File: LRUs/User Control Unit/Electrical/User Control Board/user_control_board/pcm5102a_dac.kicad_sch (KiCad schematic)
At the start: 1 part

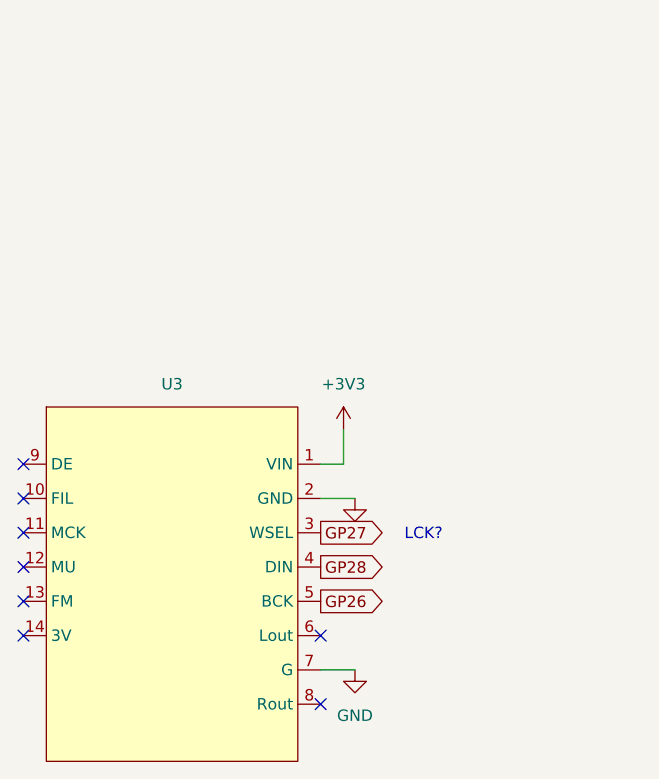
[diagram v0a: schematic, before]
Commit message: connectors and 5v buck partially done
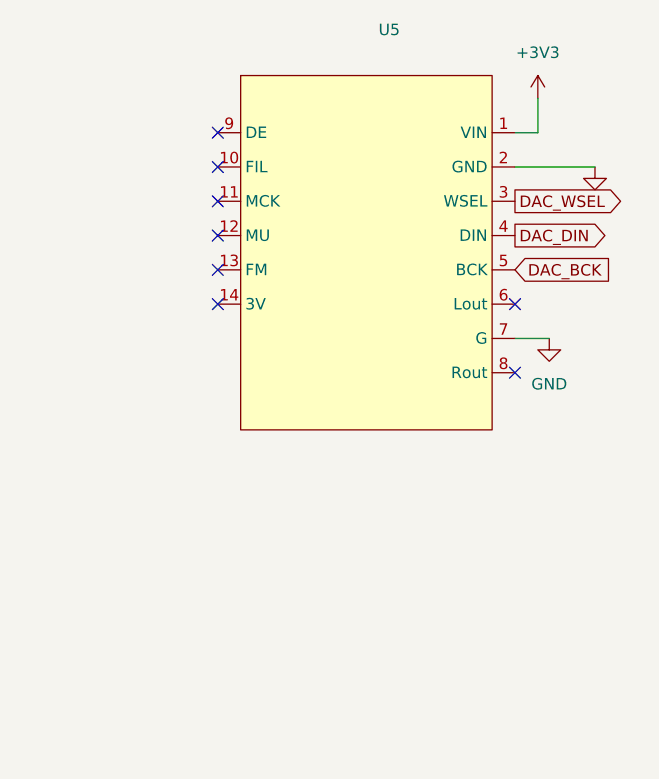
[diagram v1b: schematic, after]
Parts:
- renumbered U3 to U5
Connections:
- net GP26 renamed DAC_BCK
- net GP27 renamed DAC_WSEL
- net GP28 renamed DAC_DIN
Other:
- note removed: "LCK?"
- moved on the sheet: U5
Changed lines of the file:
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@@
 	(generator_version "10.0")
 	(paper "A4")
-	(text "LCK?"
+	(text ""
 		(exclude_from_sim no)
-		(at 132.08 136.144 0)
+		(at 159.766 104.394 0)
 		(effects
 			(font
@@
 		)
 	)
-	(text ""
-		(exclude_from_sim no)
-		(at 135.636 143.764 0)
+	(no_connect
+		(at 109.22 106.68)
+	)
+	(no_connect
+		(at 142.24 110.49)
+	)
+	(no_connect
+		(at 109.22 99.06)
+	)
+	(no_connect
+		(at 142.24 118.11)
+	)
+	(no_connect
+		(at 109.22 95.25)
+	)
+	(no_connect
+		(at 109.22 91.44)
+	)
+	(no_connect
+		(at 109.22 110.49)
+	)
+	(no_connect
+		(at 109.22 102.87)
+	)
+	(wire
+		(pts
+			(xy 144.78 91.44) (xy 142.24 91.44)
+		)
+		(stroke
+			(width 0)
+			(type default)
+		)
+	)
+	(wire
+		(pts
+			(xy 142.24 114.3) (xy 146.05 114.3)
+		)
+		(stroke
+			(width 0)
+			(type default)
+		)
+	)
+	(wire
+		(pts
+			(xy 142.24 95.25) (xy 151.13 95.25)
+		)
+		(stroke
+			(width 0)
+			(type default)
+		)
+	)
+	(wire
+		(pts
+			(xy 144.78 87.63) (xy 144.78 91.44)
+		)
+		(stroke
+			(width 0)
+			(type default)
+		)
+	)
+	(global_label "DAC_WSEL"
+		(shape output)
+		(at 142.24 99.06 0)
+		(fields_autoplaced yes)
 		(effects
 			(font
 				(size 1.27 1.27)
 			)
-		)
-	)
-	(no_connect
-		(at 87.63 143.51)
-	)
-	(no_connect
-		(at 120.65 147.32)
-	)
-	(no_connect
-		(at 87.63 135.89)
-	)
-	(no_connect
-		(at 120.65 154.94)
-	)
-	(no_connect
-		(at 87.63 132.08)
-	)
-	(no_connect
-		(at 87.63 128.27)
-	)
-	(no_connect
-		(at 87.63 147.32)
-	)
-	(no_connect
-		(at 87.63 139.7)
-	)
-	(wire
-		(pts
-			(xy 123.19 128.27) (xy 120.65 128.27)
-		)
-		(stroke
-			(width 0)
-			(type default)
-		)
-	)
-	(wire
-		(pts
-			(xy 120.65 151.13) (xy 124.46 151.13)
-		)
-		(stroke
-			(width 0)
-			(type default)
-		)
-	)
-	(wire
-		(pts
-			(xy 120.65 132.08) (xy 124.46 132.08)
-		)
-		(stroke
-			(width 0)
-			(type default)
-		)
-	)
-	(wire
-		(pts
-			(xy 123.19 124.46) (xy 123.19 128.27)
-		)
-		(stroke
-			(width 0)
-			(type default)
-		)
-	)
-	(global_label "GP27"
+			(justify left)
+		)
+		(property "Intersheetrefs" "${INTERSHEET_REFS}"
+			(at 154.6594 99.06 0)
+			(hide yes)
+			(show_name no)
+			(do_not_autoplace no)
+			(effects
+				(font
+					(size 1.27 1.27)
+				)
+				(justify left)
+			)
+		)
+	)
+	(global_label "DAC_DIN"
 		(shape output)
-		(at 120.65 135.89 0)
+		(at 142.24 102.87 0)
 		(fields_autoplaced yes)
 		(effects
@@
 		)
 		(property "Intersheetrefs" "${INTERSHEET_REFS}"
-			(at 128.5942 135.89 0)
+			(at 153.0267 102.87 0)
 			(hide yes)
 			(show_name no)
@@
 		)
 	)
-	(global_label "GP28"
-		(shape output)
-		(at 120.65 139.7 0)
+	(global_label "DAC_BCK"
+		(shape input)
+		(at 142.24 106.68 0)
 		(fields_autoplaced yes)
 		(effects
@@
 		)
 		(property "Intersheetrefs" "${INTERSHEET_REFS}"
-			(at 128.5942 139.7 0)
-			(hide yes)
-			(show_name no)
-			(do_not_autoplace no)
-			(effects
-				(font
-					(size 1.27 1.27)
-				)
-				(justify left)
-			)
-		)
-	)
-	(global_label "GP26"
-		(shape output)
-		(at 120.65 143.51 0)
-		(fields_autoplaced yes)
-		(effects
-			(font
-				(size 1.27 1.27)
-			)
-			(justify left)
-		)
-		(property "Intersheetrefs" "${INTERSHEET_REFS}"
-			(at 128.5942 143.51 0)
+			(at 153.6314 106.68 0)
 			(hide yes)
 			(show_name no)
@@
 	(symbol
 		(lib_id "power:GND")
-		(at 124.46 151.13 0)
+		(at 146.05 114.3 0)
 		(unit 1)
 		(body_style 1)
@@
 		(dnp no)
 		(fields_autoplaced yes)
-		(property "Reference" "#PWR021"
-			(at 124.46 157.48 0)
+		(property "Reference" "#PWR059"
+			(at 146.05 120.65 0)
 			(hide yes)
 			(show_name no)
@@
 		)
 		(property "Value" "GND"
-			(at 124.46 156.21 0)
+			(at 146.05 119.38 0)
 			(show_name no)
 			(do_not_autoplace no)
@@
 		)
 		(property "Footprint" ""
-			(at 124.46 151.13 0)
+			(at 146.05 114.3 0)
 			(hide yes)
 			(show_name no)
@@
 		)
 		(property "Datasheet" ""
-			(at 124.46 151.13 0)
+			(at 146.05 114.3 0)
 			(hide yes)
 			(show_name no)
@@
 		)
 		(property "Description" "Power symbol creates a global label with name \"GND\" , ground"
-			(at 124.46 151.13 0)
+			(at 146.05 114.3 0)
 			(hide yes)
 			(show_name no)
@@
 			(project "user_control_board"
 				(path "/a075224b-ddb1-4e5b-b4ec-df1a39dc2291"
-					(reference "#PWR021")
+					(reference "#PWR059")
 					(unit 1)
 				)
@@
 	(symbol
 		(lib_id "power:GND")
-		(at 124.46 132.08 0)
+		(at 151.13 95.25 0)
 		(unit 1)
 		(body_style 1)
@@
 		(dnp no)
 		(fields_autoplaced yes)
-		(property "Reference" "#PWR020"
-			(at 124.46 138.43 0)
+		(property "Reference" "#PWR058"
+			(at 151.13 101.6 0)
 			(hide yes)
 			(show_name no)
@@
 		)
 		(property "Value" "GND"
-			(at 124.46 137.16 0)
+			(at 151.13 100.33 0)
 			(hide yes)
 			(show_name no)
@@
 		)
 		(property "Footprint" ""
-			(at 124.46 132.08 0)
+			(at 151.13 95.25 0)
 			(hide yes)
 			(show_name no)
@@
 		)
 		(property "Datasheet" ""
-			(at 124.46 132.08 0)
+			(at 151.13 95.25 0)
 			(hide yes)
 			(show_name no)
@@
 		)
 		(property "Description" "Power symbol creates a global label with name \"GND\" , ground"
-			(at 124.46 132.08 0)
+			(at 151.13 95.25 0)
 			(hide yes)
 			(show_name no)
@@
 			(project "user_control_board"
 				(path "/a075224b-ddb1-4e5b-b4ec-df1a39dc2291"
-					(reference "#PWR020")
+					(reference "#PWR058")
 					(unit 1)
 				)
@@
 	(symbol
 		(lib_id "power:+3V3")
-		(at 123.19 124.46 0)
+		(at 144.78 87.63 0)
 		(unit 1)
 		(body_style 1)
@@
 		(dnp no)
 		(fields_autoplaced yes)
-		(property "Reference" "#PWR019"
-			(at 123.19 128.27 0)
+		(property "Reference" "#PWR057"
+			(at 144.78 91.44 0)
 			(hide yes)
 			(show_name no)
@@
 		)
 		(property "Value" "+3V3"
-			(at 123.19 119.38 0)
+			(at 144.78 82.55 0)
 			(show_name no)
 			(do_not_autoplace no)
@@
 		)
 		(property "Footprint" ""
-			(at 123.19 124.46 0)
+			(at 144.78 87.63 0)
 			(hide yes)
 			(show_name no)
@@
 		)
 		(property "Datasheet" ""
-			(at 123.19 124.46 0)
+			(at 144.78 87.63 0)
 			(hide yes)
 			(show_name no)
@@
 		)
 		(property "Description" "Power symbol creates a global label with name \"+3V3\""
-			(at 123.19 124.46 0)
+			(at 144.78 87.63 0)
 			(hide yes)
 			(show_name no)
@@
 			(project "user_control_board"
 				(path "/a075224b-ddb1-4e5b-b4ec-df1a39dc2291"
-					(reference "#PWR019")
+					(reference "#PWR057")
 					(unit 1)
 				)
@@
 	(symbol
 		(lib_id "symbols:PCM5102")
-		(at 102.87 148.59 0)
+		(at 127 109.22 0)
 		(unit 1)
 		(body_style 1)
@@
 		(dnp no)
 		(fields_autoplaced yes)
-		(property "Reference" "U3"
-			(at 104.14 119.38 0)
+		(property "Reference" "U5"
+			(at 128.27 80.01 0)
 			(show_name no)
 			(do_not_autoplace no)
@@
 		)
 		(property "Value" ""
-			(at 102.87 148.59 0)
+			(at 127 109.22 0)
 			(show_name no)
 			(do_not_autoplace no)
@@
 		)
 		(property "Footprint" "footprints:Adafruit PCM510x I2S DAC"
-			(at 102.87 148.59 0)
+			(at 127 109.22 0)
 			(hide yes)
 			(show_name no)
@@
 		)
 		(property "Datasheet" ""
-			(at 102.87 148.59 0)
+			(at 127 109.22 0)
 			(hide yes)
 			(show_name no)
@@
 		)
 		(property "Description" ""
-			(at 102.87 148.59 0)
+			(at 127 109.22 0)
 			(hide yes)
 			(show_name no)
@@
 			(project "user_control_board"
 				(path "/a075224b-ddb1-4e5b-b4ec-df1a39dc2291"
-					(reference "U3")
+					(reference "U5")
 					(unit 1)
 				)
